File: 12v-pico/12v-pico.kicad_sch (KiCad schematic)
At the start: 13 parts, among them J1 MERG 12v CBUS, J2 Adafruit CAN Pal, J3 Conn_01x03_Pin, J4 Conn_01x03_Pin, J5 Conn_01x20_Pin, J6 Conn_01x20_Pin, SW1 RESET, U1 LM7805_TO220

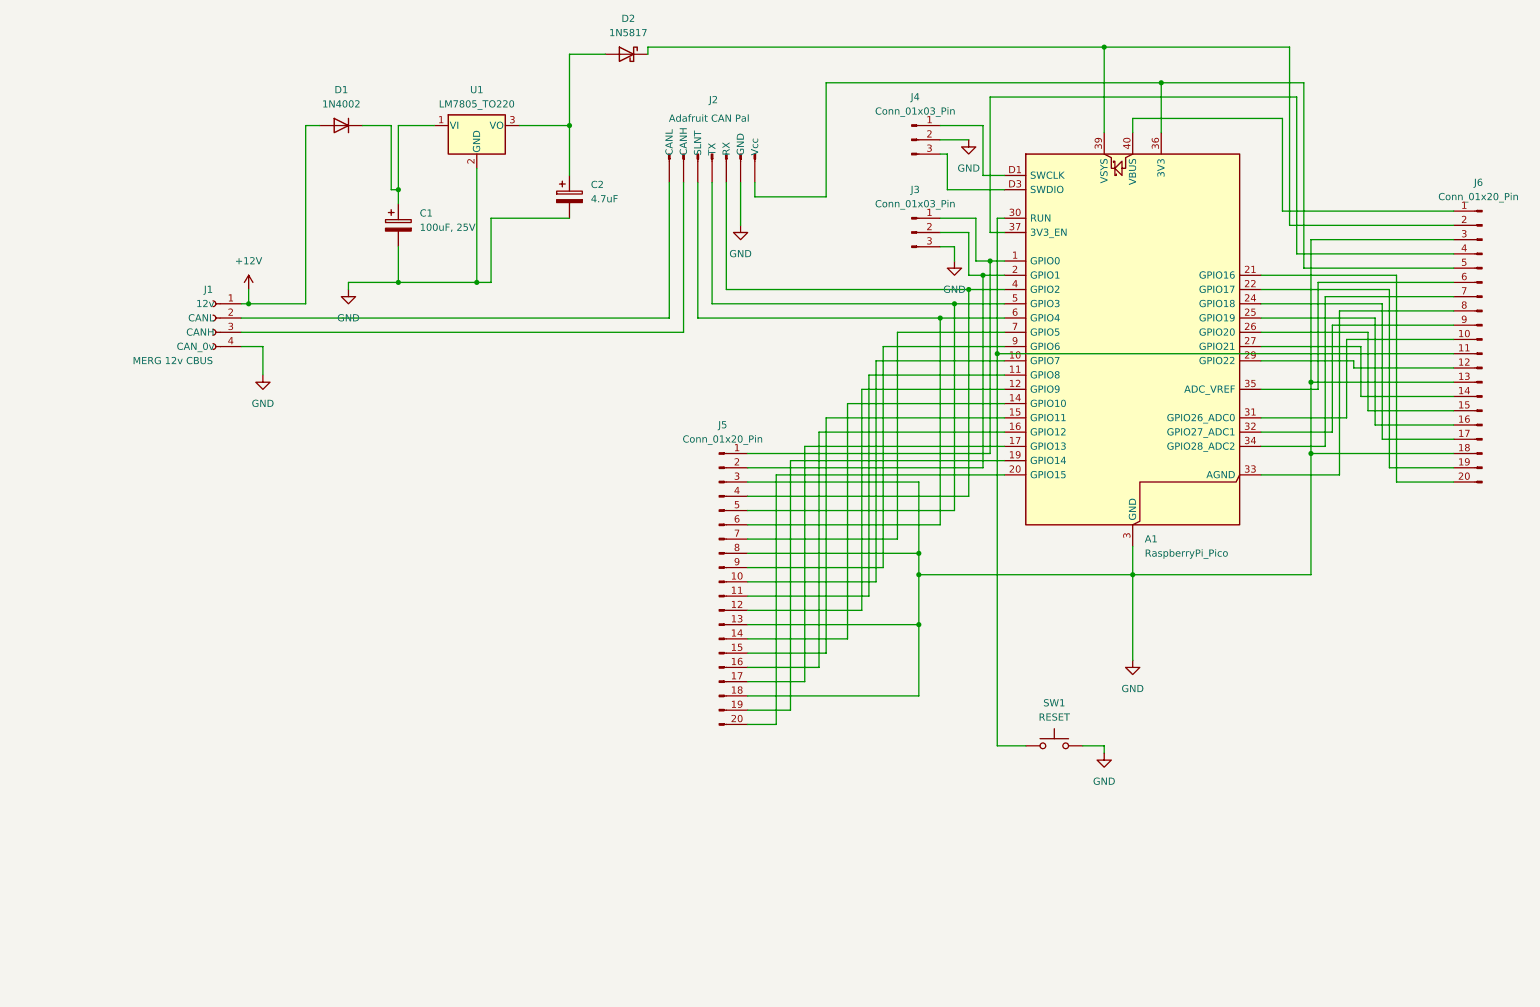
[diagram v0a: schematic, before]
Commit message: tidied up schematic
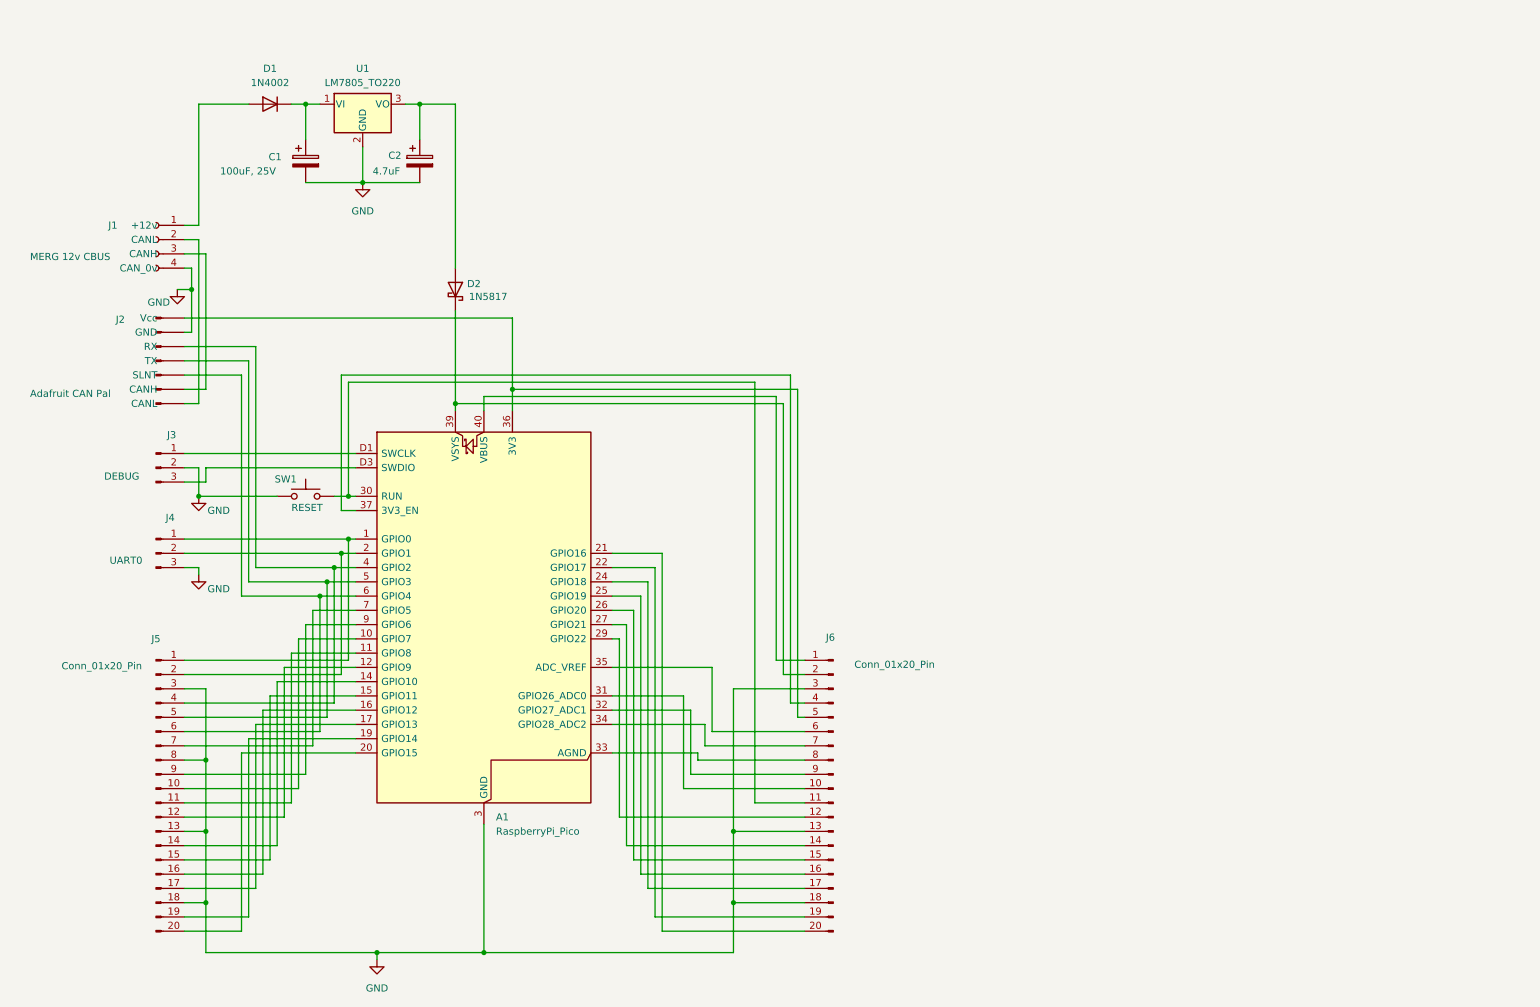
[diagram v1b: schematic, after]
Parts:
- J3: renamed from J4; value Conn_01x03_Pin -> DEBUG
- J4: renamed from J3; value Conn_01x03_Pin -> UART0
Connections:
- net GND: now also SW1.1; no longer SW1.2
- net at A1.30 (RUN), J6.11 (Pin_11): now also SW1.2; no longer SW1.1
- net +12V: no longer names the net of D1.2 (A), J1.1 (+12v)
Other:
- moved on the sheet: A1, C1, C2, D1, D2, J1, J2, J3, J4, J5, J6, SW1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
